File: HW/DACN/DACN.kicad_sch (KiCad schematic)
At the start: 0 parts

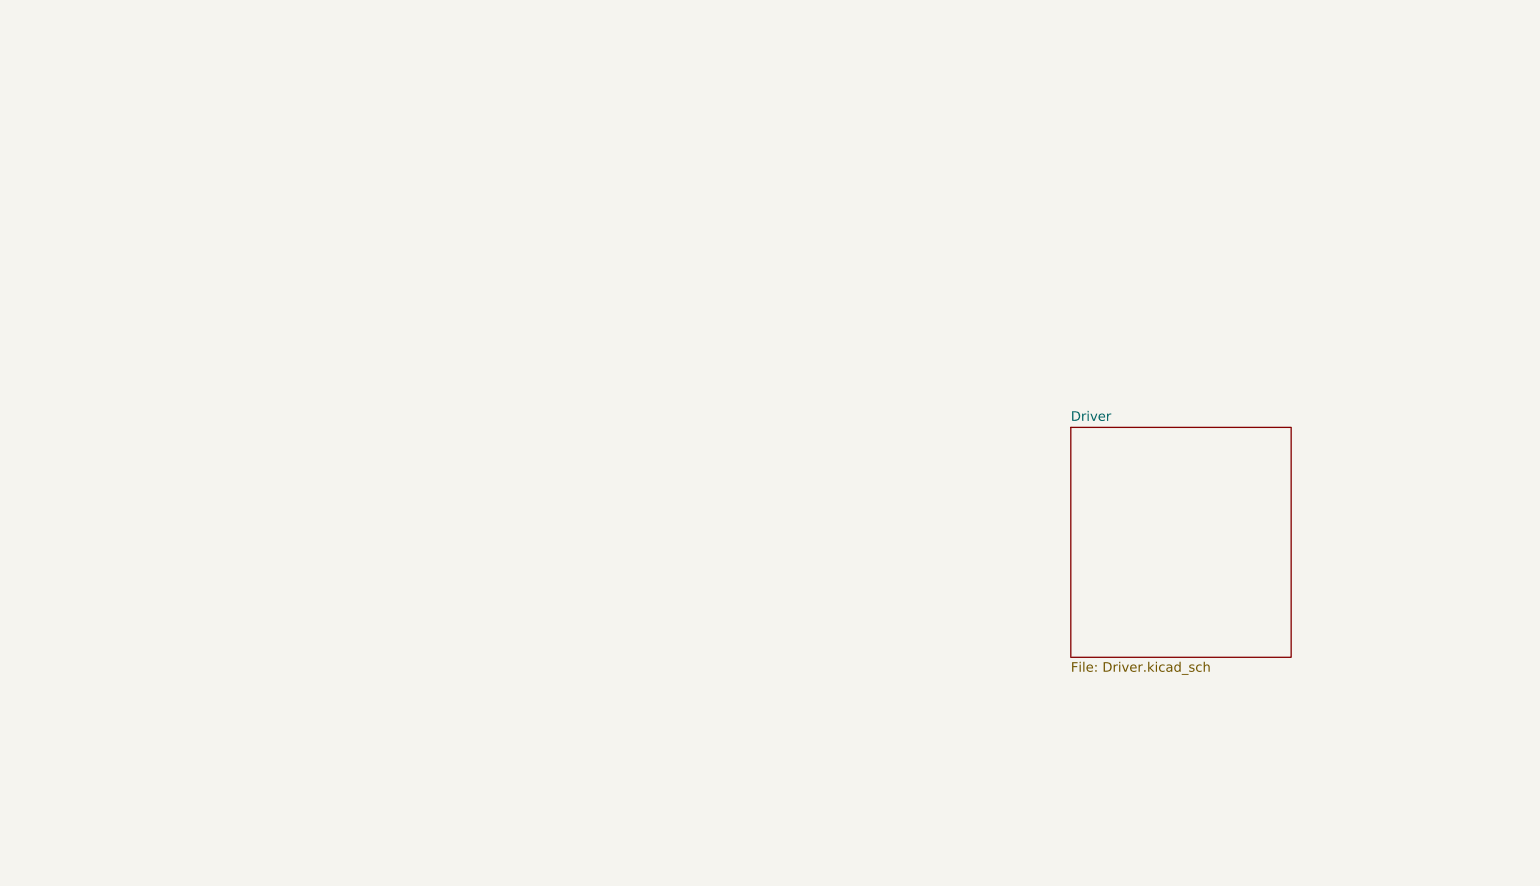
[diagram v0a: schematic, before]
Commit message: add
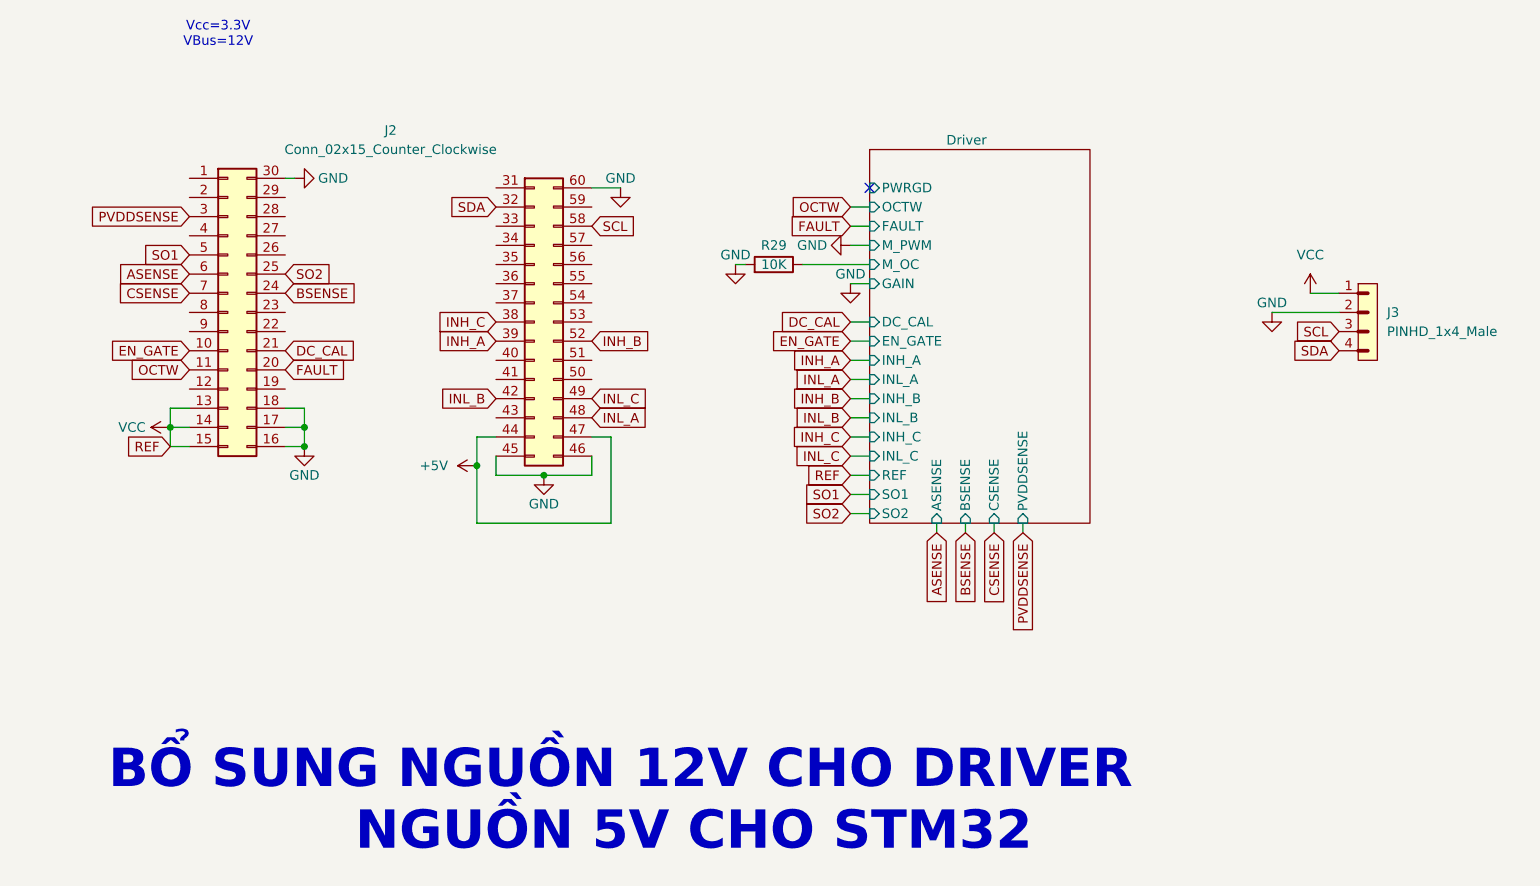
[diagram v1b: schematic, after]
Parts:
- added J2: Conn_02x15_Counter_Clockwise, Connector_PinSocket_2.54mm:Weact_STM32F405, symbol Connector_Generic:Conn_02x15_Counter_Clockwise
- added J3: PINHD_1x4_Male, Connector_PinHeader_2.54mm:PinHeader_1x04_P2.54mm_Vertical, symbol PCM_SL_Pin_Headers:PINHD_1x4_Male
- added R29: 10K, PCM_Resistor_SMD_AKL:R_0805_2012Metric, symbol PCM_Resistor_AKL:R_0805
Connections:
- new net +5V: J2.44 (Pin_44), J2.47 (Pin_47)
- new net ASENSE: J2.6 (Pin_6)
- new net BSENSE: J2.24 (Pin_24)
- new net CSENSE: J2.7 (Pin_7)
- new net DC_CAL: J2.21 (Pin_21)
- new net Driver/M_OC: R29.2
- new net EN_GATE: J2.10 (Pin_10)
- new net FAULT: J2.20 (Pin_20)
- new net GND: J2.16 (Pin_16), J2.17 (Pin_17), J2.18 (Pin_18), J2.30 (Pin_30), J2.45 (Pin_45), J2.46 (Pin_46), J2.60 (Pin_60), J3.2, R29.1
- new net INH_A: J2.39 (Pin_39)
- new net INH_B: J2.52 (Pin_52)
- new net INH_C: J2.38 (Pin_38)
- new net INL_A: J2.48 (Pin_48)
- new net INL_B: J2.42 (Pin_42)
- new net INL_C: J2.49 (Pin_49)
- new net OCTW: J2.11 (Pin_11)
- new net PVDDSENSE: J2.3 (Pin_3)
- new net SCL: J2.58 (Pin_58), J3.3
- new net SDA: J2.32 (Pin_32), J3.4
- new net SO1: J2.5 (Pin_5)
- new net SO2: J2.25 (Pin_25)
- new net VCC: J2.13 (Pin_13), J2.14 (Pin_14), J2.15 (Pin_15), J3.1
- no-connect marks 0 -> 1
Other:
- sheet Driver ports: added ASENSE, BSENSE, CSENSE, DC_CAL, EN_GATE, FAULT, GAIN, INH_A, INH_B, INH_C, INL_A, INL_B, INL_C, M_OC, M_PWM, OCTW, PVDDSENSE, PWRGD, REF, SO1, SO2; removed none
- note added: "BỔ SUNG NGUỒN 12V CHO DRIVER NGUỒN 5V CHO STM32"
- note added: "Vcc=3.3V VBus=12V"
